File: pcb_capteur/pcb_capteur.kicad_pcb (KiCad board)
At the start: 2 copper layers, 68.6 x 53.3 mm, 22 parts, among them P1 Power, P2 Analog, P3 Digital, P4 Digital, P5 CONN_01X01, P6 CONN_01X01, P7 CONN_01X01, P8 CONN_01X01, U1 OLED-I2C, U2 LTC1050, U3 HC-05, U4 KY-040

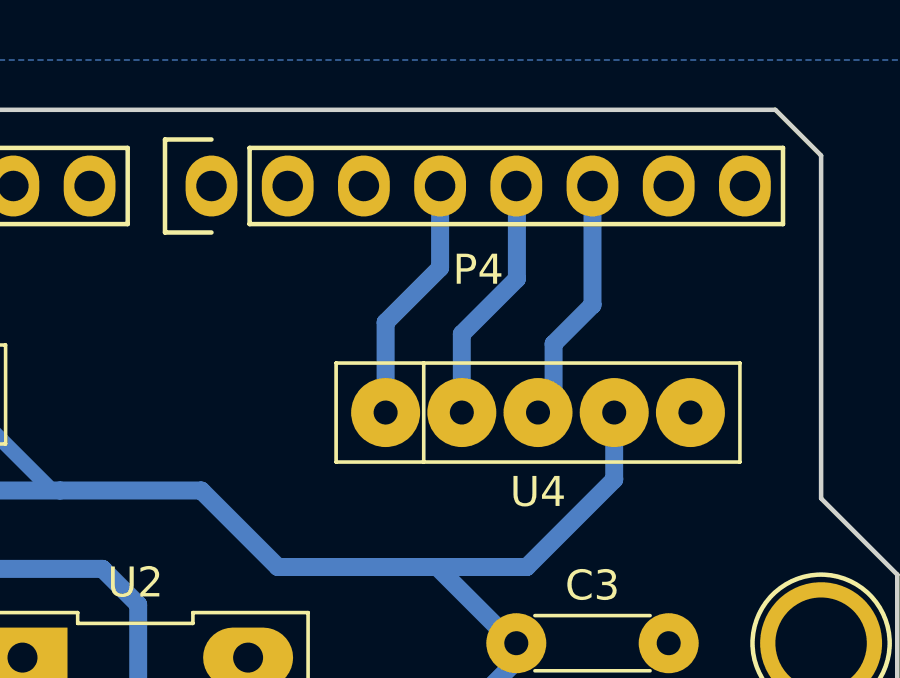
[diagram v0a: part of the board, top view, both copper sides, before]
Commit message: Fourth commit
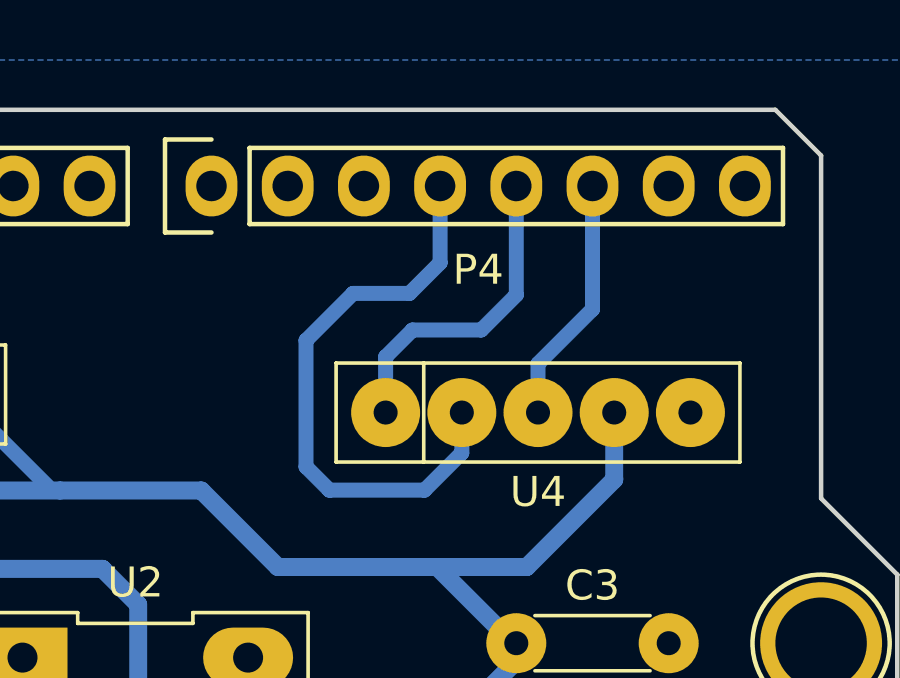
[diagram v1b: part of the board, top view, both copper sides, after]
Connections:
- P4 pad 4: CLK -> DATA
- P4 pad 5: DATA -> CLK
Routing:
- net DATA: track 8.32 -> 19.7 mm
- net CLK: track 8.30 -> 10.7 mm
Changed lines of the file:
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@@
       (net 17 "/5(**)") (pinfunction "Pin_3") (pintype "passive"))
     (pad "4" thru_hole oval locked (at 7.62 0) (size 1.7272 2.032) (drill 1.016) (layers *.Cu *.Mask "F.SilkS")
-      (net 30 "CLK") (pinfunction "Pin_4") (pintype "passive"))
+      (net 29 "DATA") (pinfunction "Pin_4") (pintype "passive"))
     (pad "5" thru_hole oval locked (at 10.16 0) (size 1.7272 2.032) (drill 1.016) (layers *.Cu *.Mask "F.SilkS")
-      (net 29 "DATA") (pinfunction "Pin_5") (pintype "passive"))
+      (net 30 "CLK") (pinfunction "Pin_5") (pintype "passive"))
     (pad "6" thru_hole oval locked (at 12.7 0) (size 1.7272 2.032) (drill 1.016) (layers *.Cu *.Mask "F.SilkS")
       (net 28 "SW") (pinfunction "Pin_6") (pintype "passive"))
@@
   (segment (start 140.583881 82.51496) (end 140.583881 80.015119) (width 0.5) (layer "B.Cu") (net 26))
   (segment (start 140.583881 80.015119) (end 145.034 75.565) (width 0.5) (layer "B.Cu") (net 26))
-  (segment (start 167.602183 83.116529) (end 168.121292 82.59742) (width 0.6) (layer "B.Cu") (net 28))
-  (segment (start 168.121292 80.827161) (end 169.418 79.530453) (width 0.6) (layer "B.Cu") (net 28))
-  (segment (start 168.121292 82.59742) (end 168.121292 80.827161) (width 0.6) (layer "B.Cu") (net 28))
-  (segment (start 169.418 79.530453) (end 169.418 75.565) (width 0.6) (layer "B.Cu") (net 28))
-  (segment (start 166.897152 78.661374) (end 166.897152 75.584152) (width 0.6) (layer "B.Cu") (net 29))
-  (segment (start 166.897152 75.584152) (end 166.878 75.565) (width 0.6) (layer "B.Cu") (net 29))
-  (segment (start 165.062183 83.116529) (end 165.062183 80.496343) (width 0.6) (layer "B.Cu") (net 29))
-  (segment (start 165.062183 80.496343) (end 166.897152 78.661374) (width 0.6) (layer "B.Cu") (net 29))
-  (segment (start 162.522183 80.110471) (end 164.338 78.294654) (width 0.6) (layer "B.Cu") (net 30))
-  (segment (start 164.338 78.294654) (end 164.338 75.565) (width 0.6) (layer "B.Cu") (net 30))
-  (segment (start 162.522183 83.116529) (end 162.522183 80.110471) (width 0.6) (layer "B.Cu") (net 30))
+  (segment (start 167.602183 81.490184) (end 169.418 79.674367) (width 0.5) (layer "B.Cu") (net 28))
+  (segment (start 169.418 79.674367) (end 169.418 75.565) (width 0.5) (layer "B.Cu") (net 28))
+  (segment (start 167.602183 83.116529) (end 167.602183 81.490184) (width 0.5) (layer "B.Cu") (net 28))
+  (segment (start 164.338 78.125) (end 164.338 75.565) (width 0.5) (layer "B.Cu") (net 29))
+  (segment (start 165.062183 84.460817) (end 163.818 85.705) (width 0.5) (layer "B.Cu") (net 29))
+  (segment (start 165.062183 83.116529) (end 165.062183 84.460817) (width 0.5) (layer "B.Cu") (net 29))
+  (segment (start 160.648 85.705) (end 159.868 84.925) (width 0.5) (layer "B.Cu") (net 29))
+  (segment (start 161.438 79.145) (end 163.318 79.145) (width 0.5) (layer "B.Cu") (net 29))
+  (segment (start 159.868 84.925) (end 159.868 80.715) (width 0.5) (layer "B.Cu") (net 29))
+  (segment (start 159.868 80.715) (end 161.438 79.145) (width 0.5) (layer "B.Cu") (net 29))
+  (segment (start 163.818 85.705) (end 160.648 85.705) (width 0.5) (layer "B.Cu") (net 29))
+  (segment (start 163.318 79.145) (end 164.338 78.125) (width 0.5) (layer "B.Cu") (net 29))
+  (segment (start 165.708 80.365) (end 166.878 79.195) (width 0.5) (layer "B.Cu") (net 30))
+  (segment (start 166.878 79.195) (end 166.878 75.565) (width 0.5) (layer "B.Cu") (net 30))
+  (segment (start 166.897152 75.584152) (end 166.878 75.565) (width 0.6) (layer "B.Cu") (net 30))
+  (segment (start 163.418 80.365) (end 165.708 80.365) (width 0.5) (layer "B.Cu") (net 30))
+  (segment (start 162.522183 83.116529) (end 162.522183 81.260817) (width 0.5) (layer "B.Cu") (net 30))
+  (segment (start 162.522183 81.260817) (end 163.418 80.365) (width 0.5) (layer "B.Cu") (net 30))
   (segment (start 128.778 114.935) (end 126.123885 114.935) (width 0.6) (layer "B.Cu") (net 36))
   (segment (start 116.078 104.889115) (end 116.078 98.635) (width 0.6) (layer "B.Cu") (net 36))
